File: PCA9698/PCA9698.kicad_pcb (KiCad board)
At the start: 4 copper layers, 8 parts, among them U1 WPMDH1100501S, U2 PCA9698, U3 ADS7828, U4 LTC6802-2, U5 SC18IS602B, U6 LTC6802-2, U7 LTC6802-2, U8 LTC6802-2

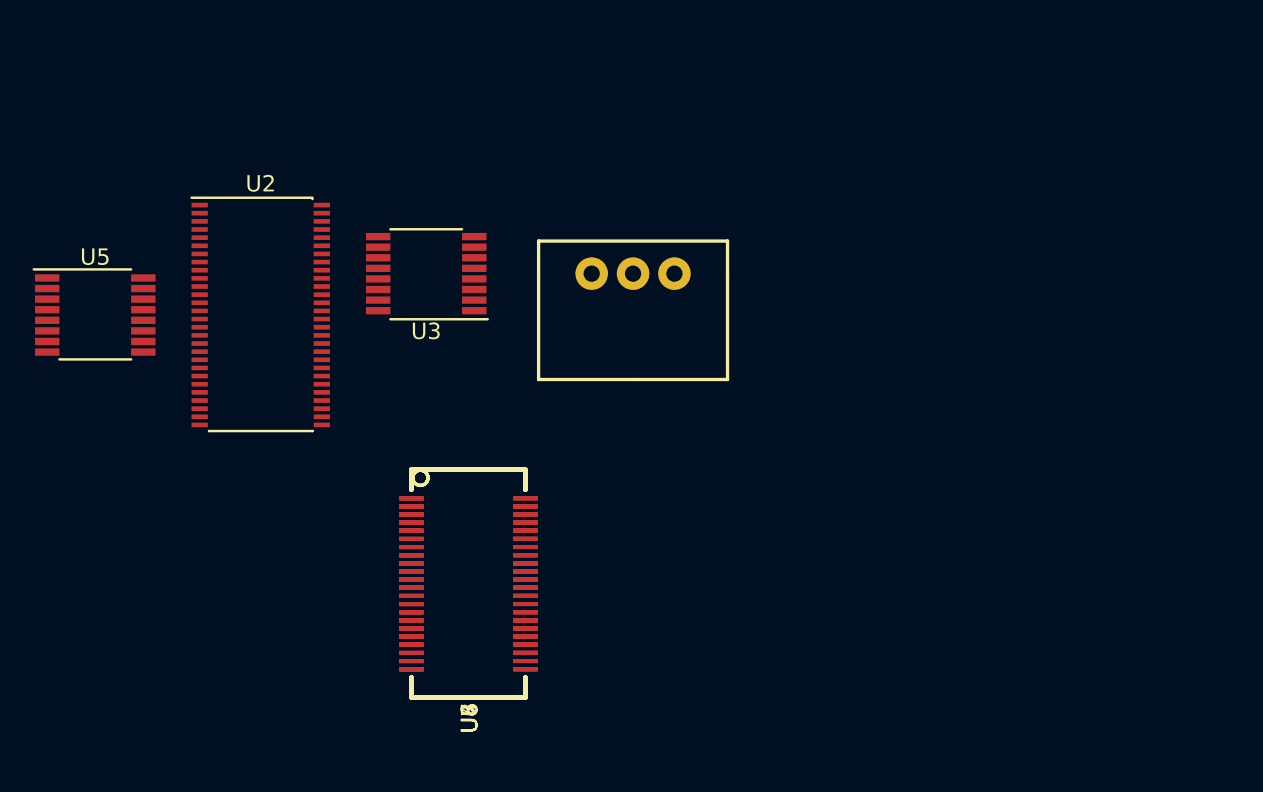
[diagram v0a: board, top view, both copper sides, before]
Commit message: test
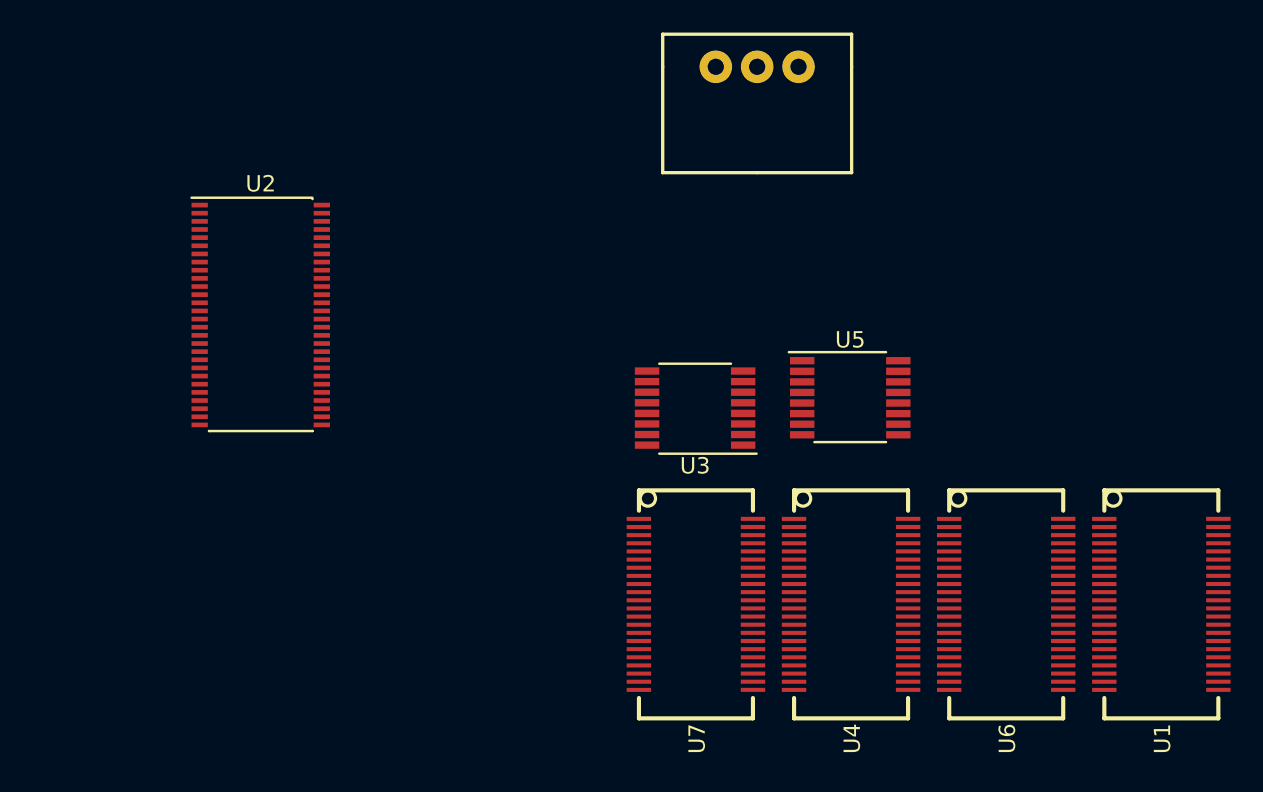
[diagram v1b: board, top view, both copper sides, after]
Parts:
- U1: value WPMDH1100501S -> LTC6802-2; footprint we:WPMDH1100xx1S -> KiCad-Dev:SSOP-44
- U8: value LTC6802-2 -> WPMDH1100331S; footprint KiCad-Dev:SSOP-44 -> we:WPMDH1100xx1S
- moved U5 46.6 mm to (203.8, 81.3)
- moved U1 38.2 mm to (222.9, 94.0)
- moved U8 36.4 mm to (198.1, 61.0)
- moved U6 33.0 mm to (213.4, 94.0)
- moved U4 23.5 mm to (203.8, 94.0)
- moved U3 18.5 mm to (194.3, 81.9)
- moved U7 14.0 mm to (194.3, 94.0)
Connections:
- U1 pad 1: (no net) -> +3V3
- U6 pad 1: (no net) -> +3V3
- U8 pad 2: (no net) -> GND
- U8 pad 3: (no net) -> +3V3
